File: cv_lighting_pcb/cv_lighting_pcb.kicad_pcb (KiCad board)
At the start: 2 copper layers, 81.3 x 76.2 mm, 27 parts, among them Q1 2N3906, U1 Current Driver, U2 Camera Input, U3 VO617A, U4 Barrel Jack

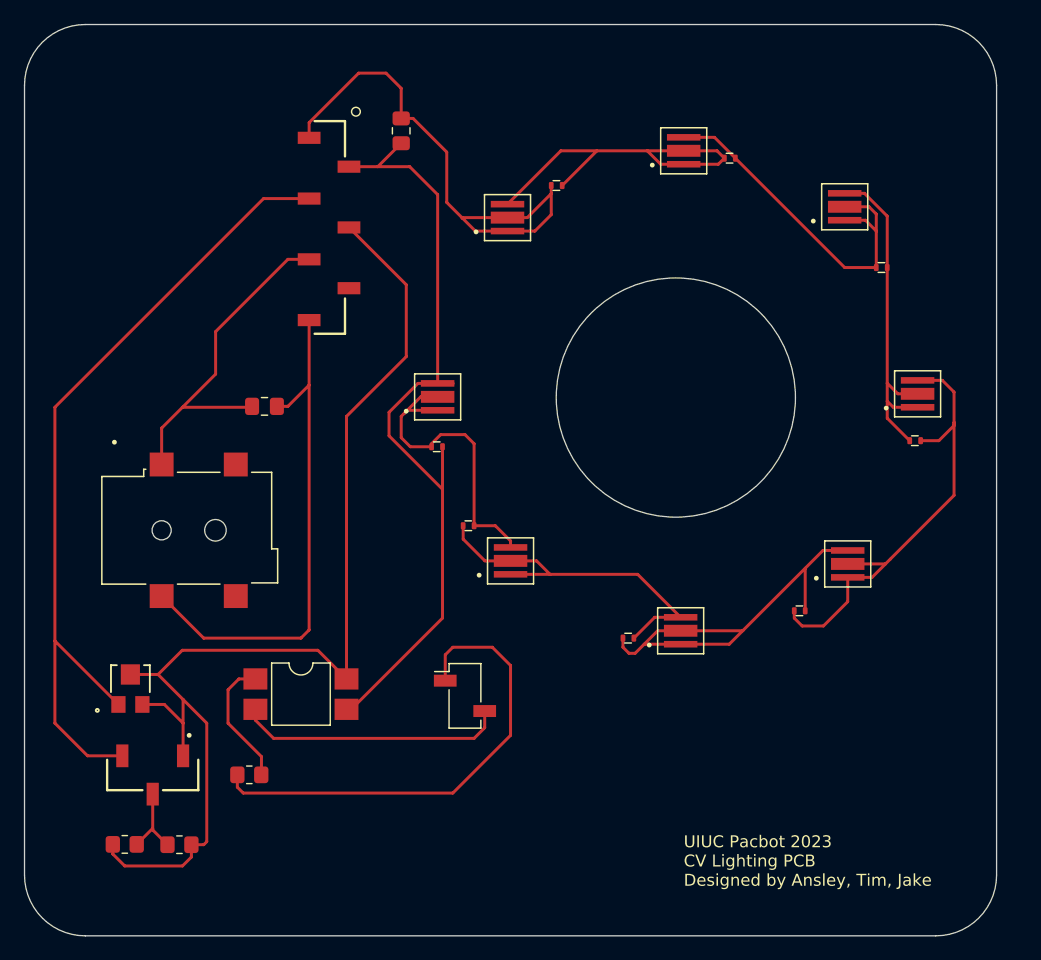
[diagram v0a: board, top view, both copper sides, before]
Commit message: changes to lighting pcb
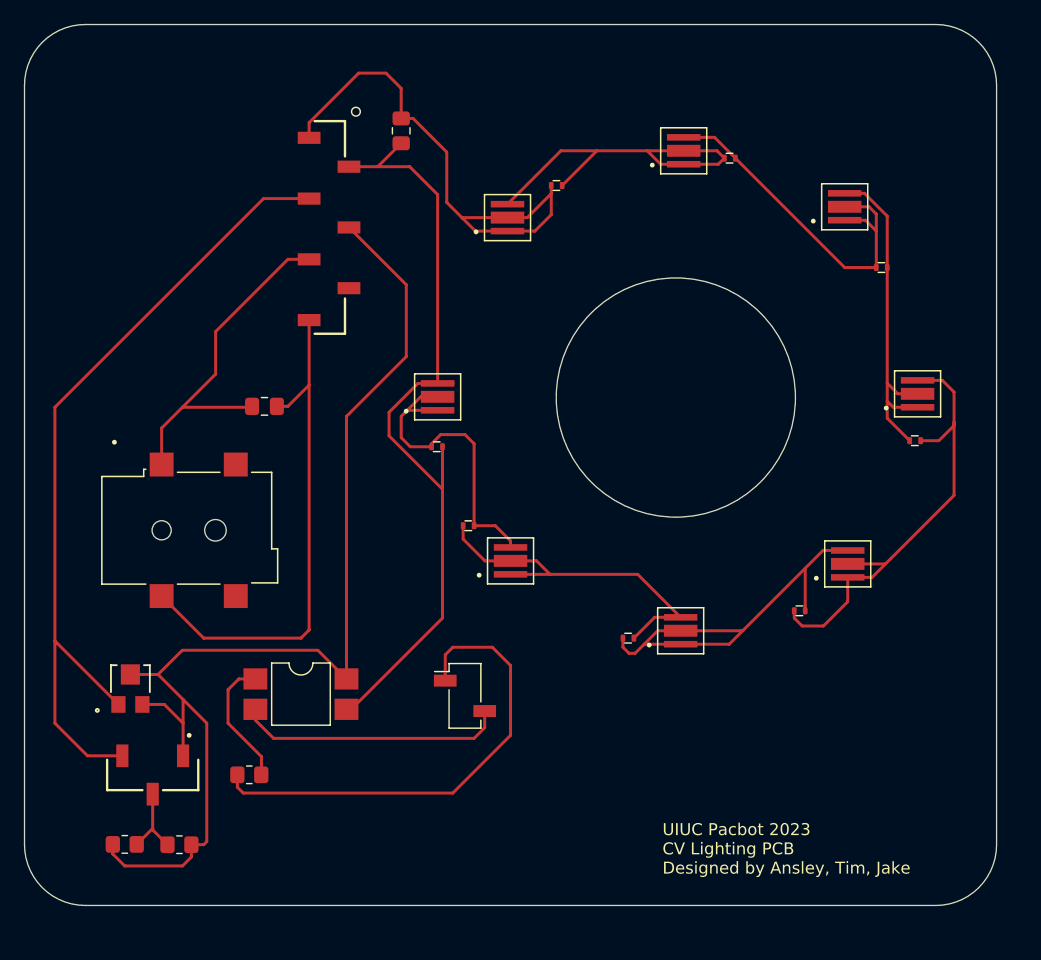
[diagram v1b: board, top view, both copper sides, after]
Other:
- board size 81.3 x 76.2 mm -> 81.3 x 73.7 mm
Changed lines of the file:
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@@
       (net 12 "Net-(Q1-C)") (pinfunction "C") (pintype "passive") (solder_mask_margin 0.102))
   )
+  (gr_arc (start 106.68 124.46) (mid 103.087898 122.972102) (end 101.6 119.38)
+    (stroke (width 0.1) (type default)) (layer "Edge.Cuts"))
   (gr_circle (center 167.5892 81.9912) (end 167.5892 81.9912)
     (stroke (width 0.1) (type default)) (fill none) (layer "Edge.Cuts"))
-  (gr_line (start 182.88 55.88) (end 182.88 121.92)
+  (gr_line (start 182.88 55.88) (end 182.88 119.38)
     (stroke (width 0.1) (type default)) (layer "Edge.Cuts"))
   (gr_line (start 106.68 50.8) (end 177.8 50.8)
@@
   (gr_arc (start 101.6 55.88) (mid 103.087898 52.287898) (end 106.68 50.8)
     (stroke (width 0.1) (type default)) (layer "Edge.Cuts"))
-  (gr_line (start 101.6 121.92) (end 101.6 55.88)
+  (gr_line (start 101.6 119.38) (end 101.6 55.88)
     (stroke (width 0.1) (type default)) (layer "Edge.Cuts"))
-  (gr_line (start 177.8 127) (end 106.68 127)
+  (gr_line (start 177.8 124.46) (end 106.68 124.46)
     (stroke (width 0.1) (type default)) (layer "Edge.Cuts"))
   (gr_circle (center 156.061042 81.9912) (end 166.061047 81.9912)
     (stroke (width 0.1) (type default)) (fill none) (layer "Edge.Cuts"))
-  (gr_arc (start 106.68 127) (mid 103.087898 125.512102) (end 101.6 121.92)
+  (gr_arc (start 182.88 119.38) (mid 181.392102 122.972102) (end 177.8 124.46)
     (stroke (width 0.1) (type default)) (layer "Edge.Cuts"))
   (gr_arc (start 177.8 50.8) (mid 181.392102 52.287898) (end 182.88 55.88)
     (stroke (width 0.1) (type default)) (layer "Edge.Cuts"))
-  (gr_arc (start 182.88 121.92) (mid 181.392102 125.512102) (end 177.8 127)
-    (stroke (width 0.1) (type default)) (layer "Edge.Cuts"))
   (gr_circle (center 156.061042 81.9912) (end 176.381042 81.9912)
     (stroke (width 0.1) (type default)) (fill none) (layer "F.Fab"))
-  (gr_text "UIUC Pacbot 2023\nCV Lighting PCB\nDesigned by Ansley, Tim, Jake" (at 156.718 122.936) (layer "F.SilkS")
+  (gr_text "UIUC Pacbot 2023\nCV Lighting PCB\nDesigned by Ansley, Tim, Jake" (at 154.94 121.92) (layer "F.SilkS")
     (effects (font (size 1 1) (thickness 0.15)) (justify left bottom))
   )
